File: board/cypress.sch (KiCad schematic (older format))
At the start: 48 parts, among them J1 USB_MICRO_B, U1 CY7C68013A, U4 M25P16, X1 CRYSTAL

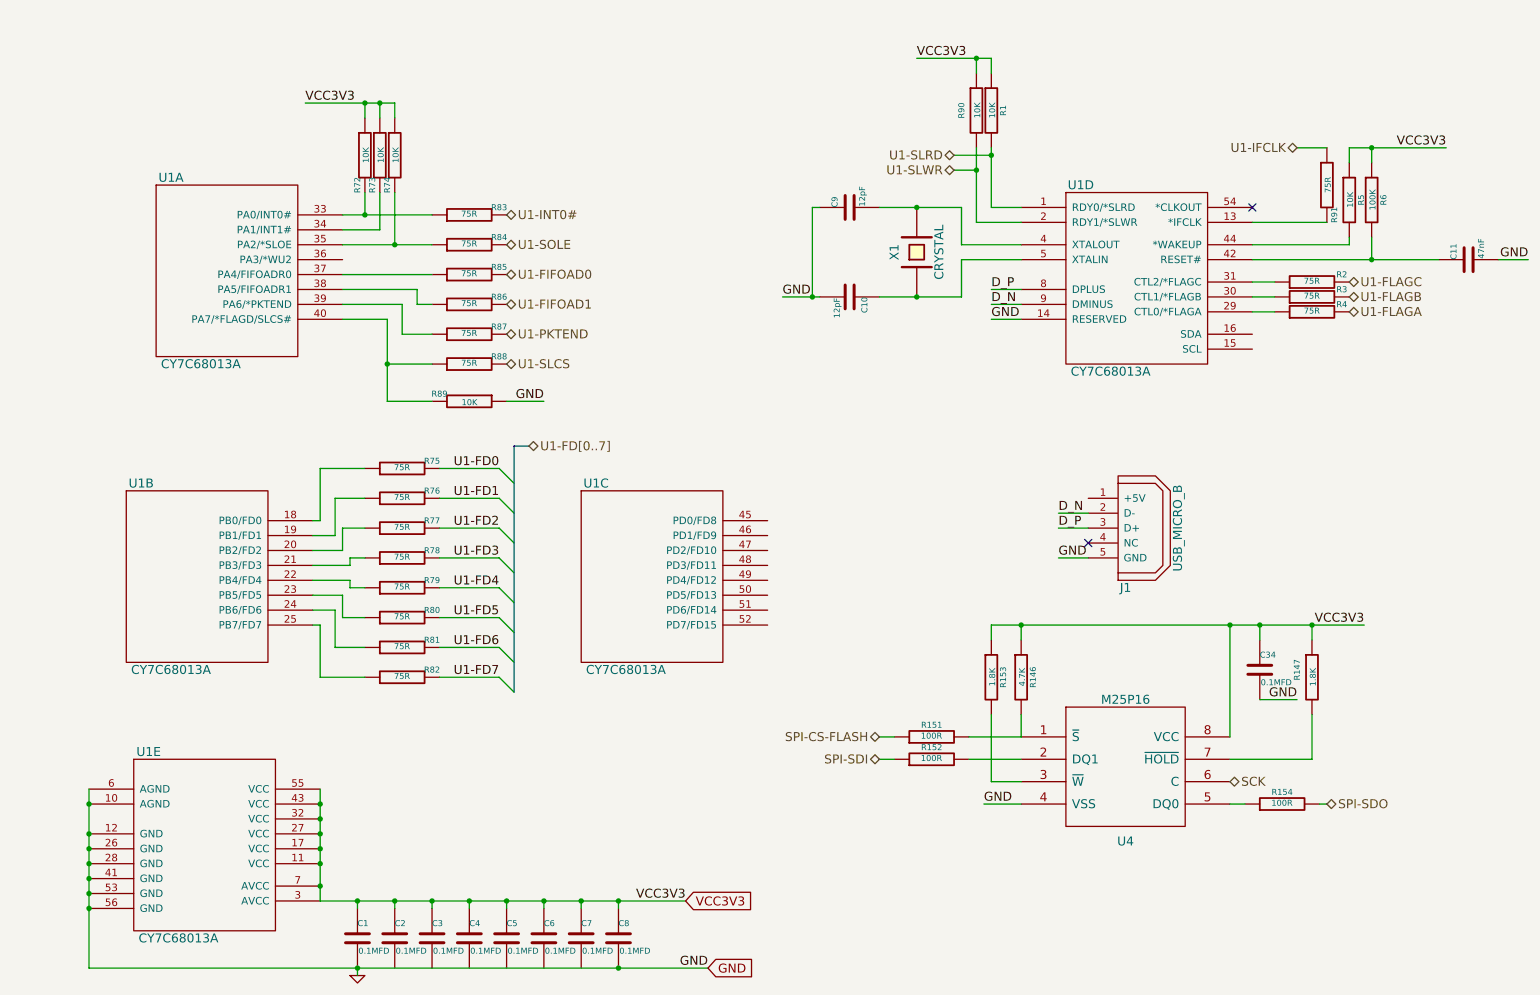
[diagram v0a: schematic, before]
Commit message: Issue #336
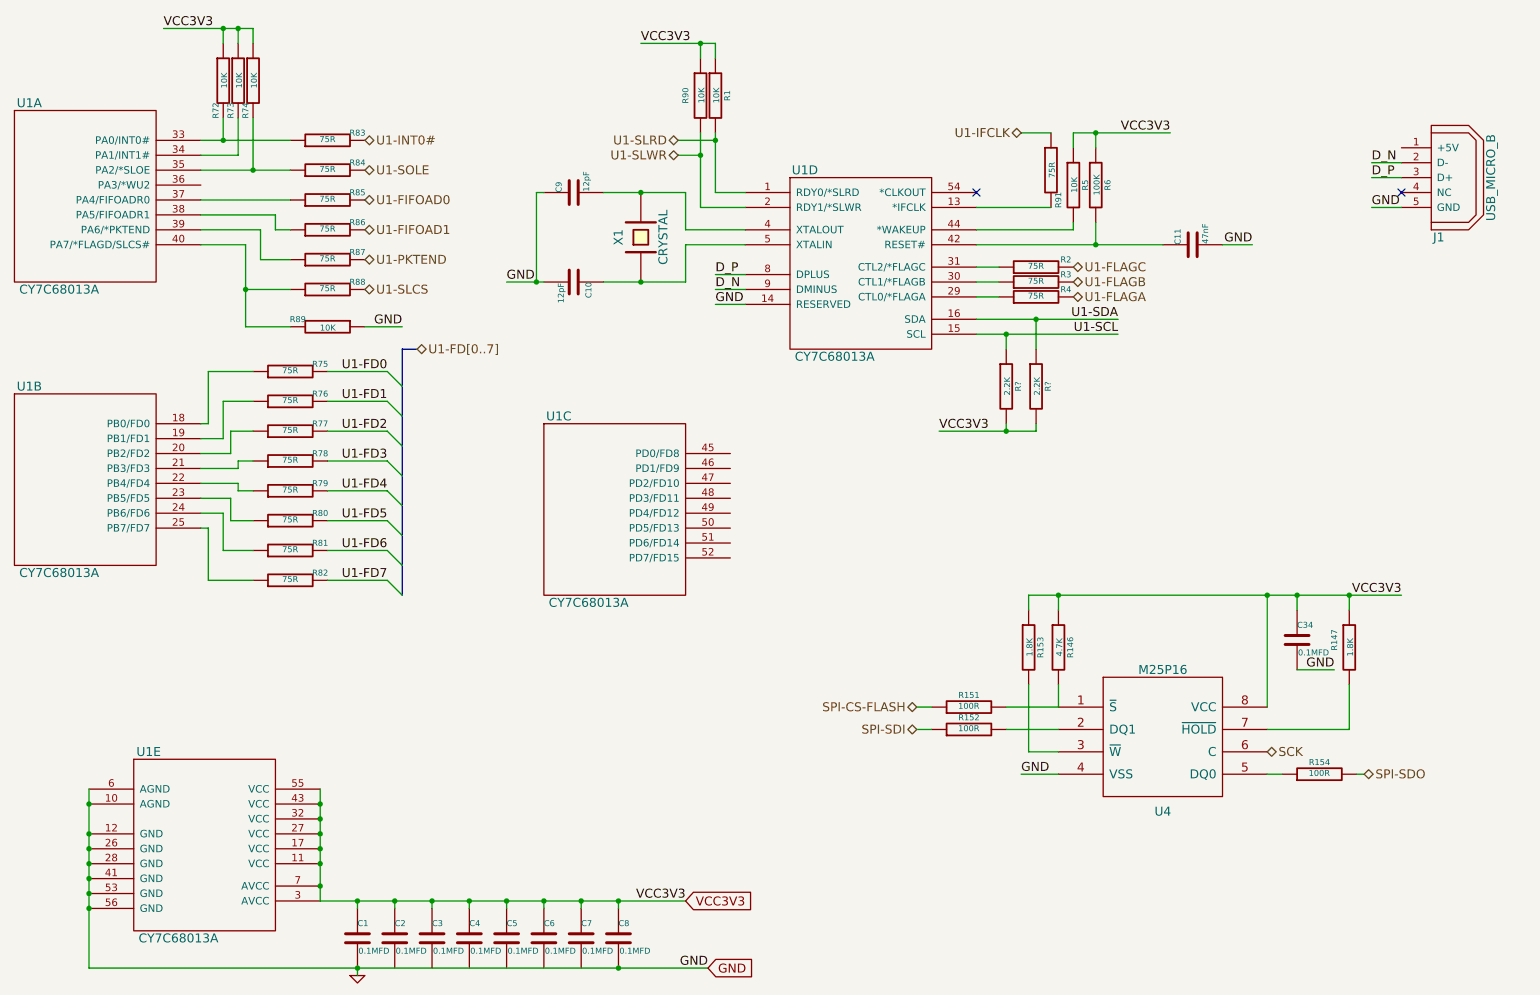
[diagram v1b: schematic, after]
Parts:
- added R? (x2): 2.2K, ~, symbol R
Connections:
- net VCC3V3: now also R?.2, R?.2
- net U1-SCL: now reaches U1.15 (SCL)
- net U1-SCL: now also R?.1
- net U1-SDA: now reaches U1.16 (SDA)
- net U1-SDA: now also R?.1
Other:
- moved on the sheet: C10, C11, C34, C9, J1, R1, R146, R147, R151, R152, R153, R154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
